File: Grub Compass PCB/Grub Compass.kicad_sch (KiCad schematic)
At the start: 28 parts, among them J1 USB_C_Receptacle_USB2.0_16P, M1 Motor_Servo, Q1 IRLML6302TRPBF, SW1 TS-1088-AR02016, SW2 TS-1088-AR02016, U1 ESP32-C3-WROOM-02, U2 AMS1117-3.3, U3 BC-4-3PD, U4 MCP73831-2-OT

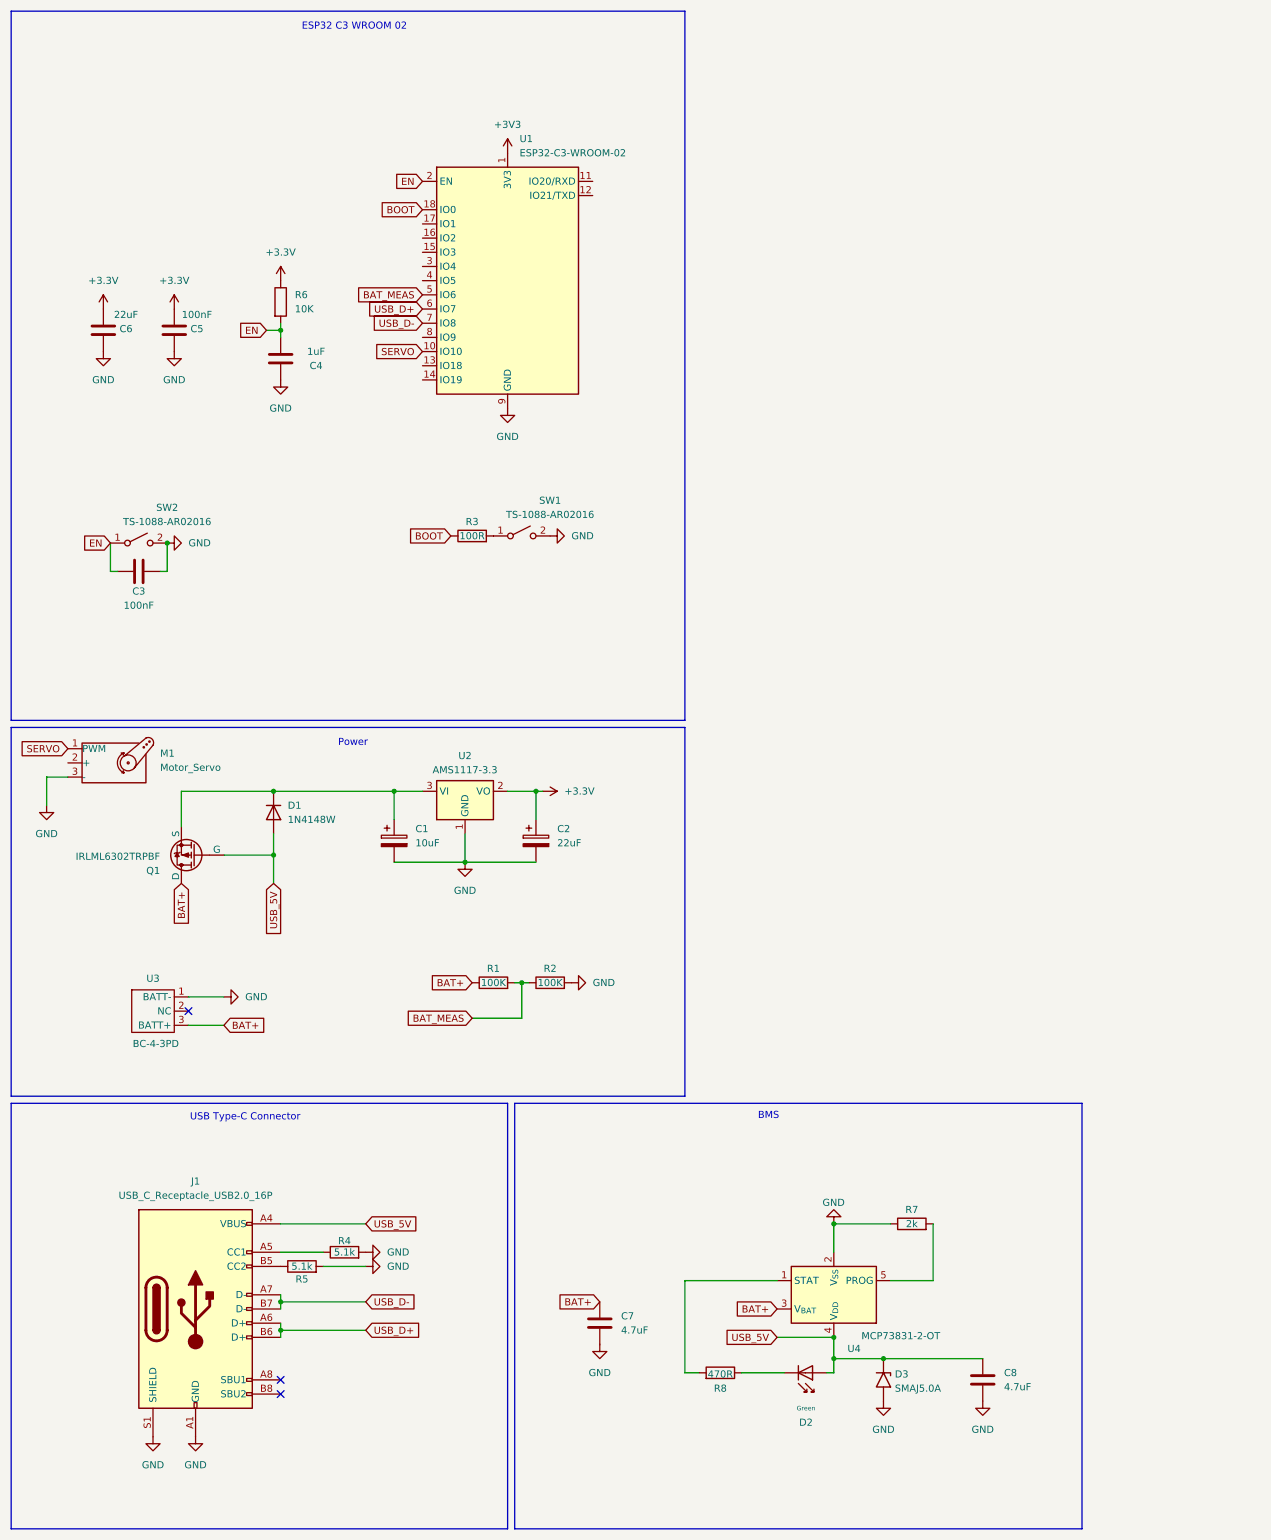
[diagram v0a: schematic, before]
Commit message: Day 3 update
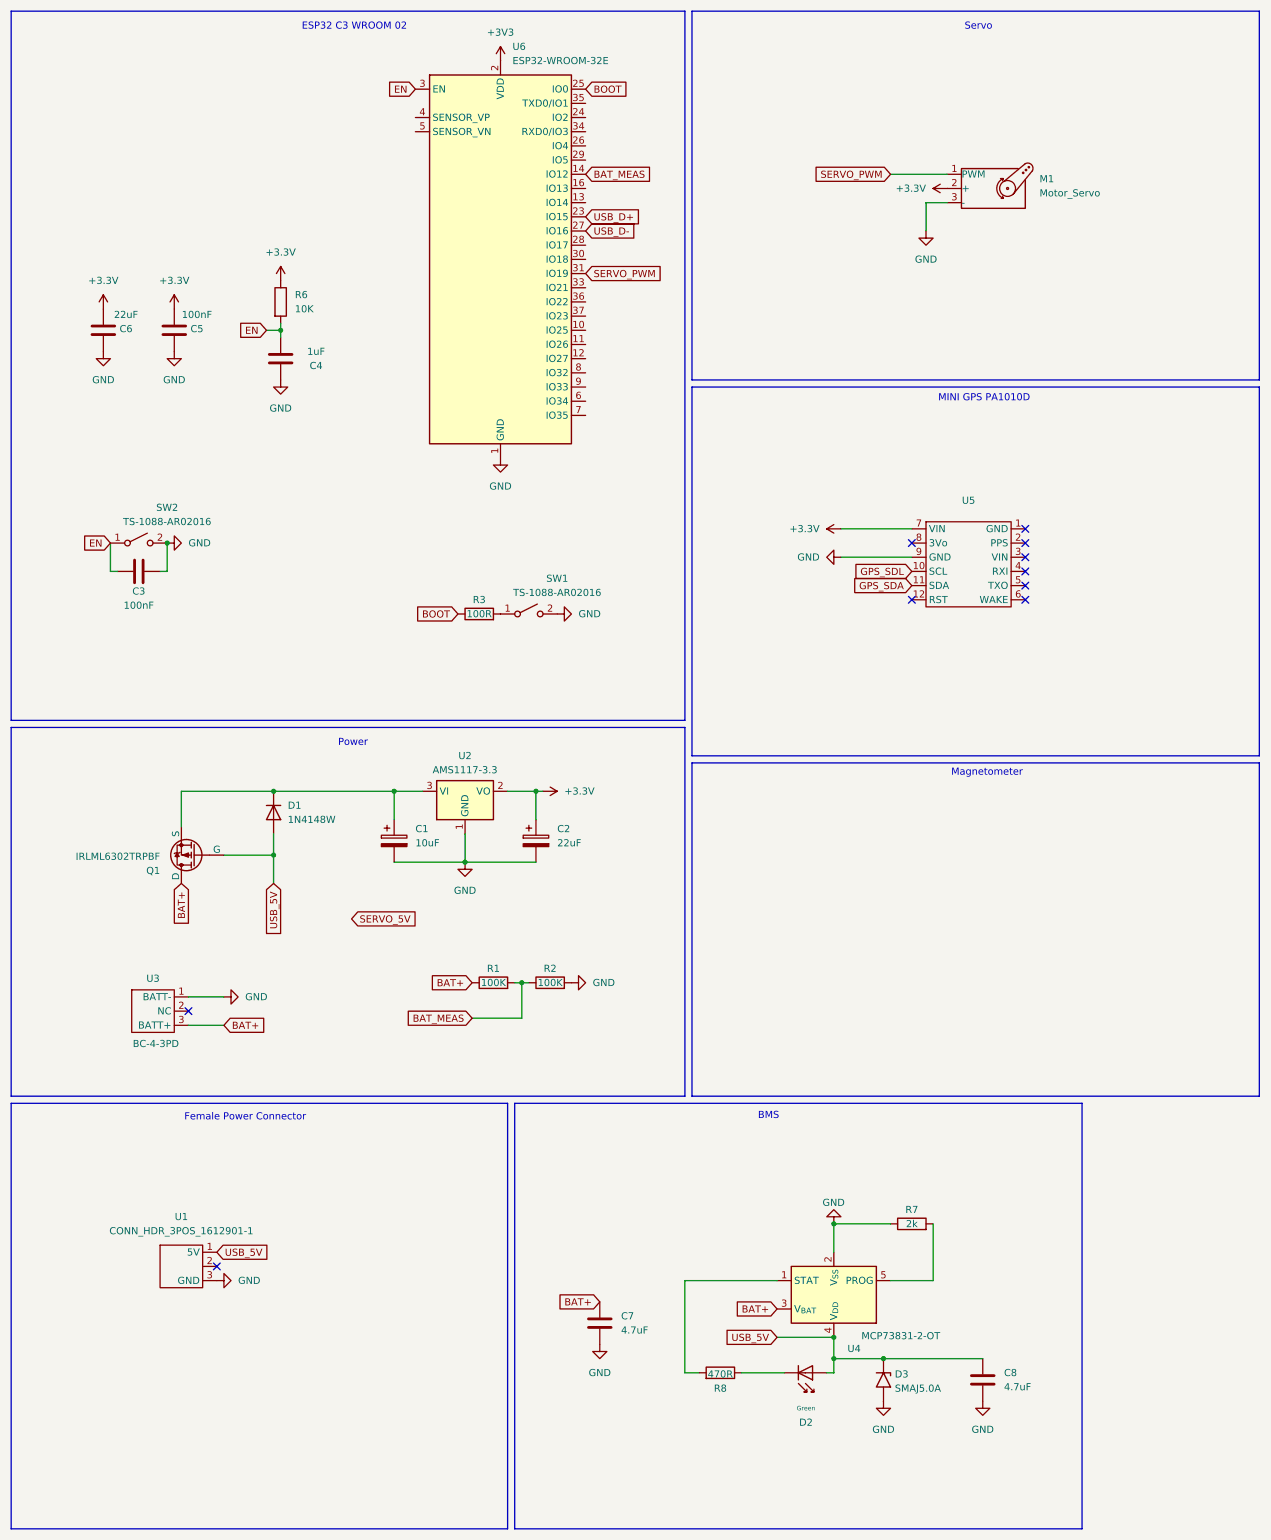
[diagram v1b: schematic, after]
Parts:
- removed J1: USB_C_Receptacle_USB2.0_16P, symbol Connector:USB_C_Receptacle_USB2.0_16P
- removed R4, R5: 5.1k, Resistor_SMD:R_0201_0603Metric, symbol Device:R
- removed U1: ESP32-C3-WROOM-02, RF_Module:ESP32-C3-WROOM-02, symbol RF_Module:ESP32-C3-WROOM-02
- added U1: CONN_HDR_3POS_1612901-1, symbol grubCompass:CONN_HDR_3POS_1612898-1
- added U5: ~, symbol grubCompass:MINI_GPS_PA1010D_STEMMA_QT
- added U6: ESP32-WROOM-32E, RF_Module:ESP32-WROOM-32D, symbol RF_Module:ESP32-WROOM-32E
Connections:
- net +3.3V: now also M1.2 (+), U5.7 (VIN)
- net +3V3: now also U6.2 (VDD)
- net BAT_MEAS: now also U6.14 (IO12)
- net BOOT: now also U6.25 (IO0)
- net EN: now also U6.3 (EN)
- net GND: now also U1.3 (GND), U5.9 (GND), U6.1 (GND), U6.15 (GND), U6.38 (GND), U6.39 (GND)
- net USB_5V: now also U1.1 (5V)
- net USB_D+: now also U6.23 (IO15)
- net USB_D-: now also U6.27 (IO16)
- net SERVO renamed SERVO_PWM
- net SERVO_PWM: now also U6.31 (IO19)
- new net GPS_SDA: U5.11 (SDA)
- new net GPS_SDL: U5.10 (SCL)
- no-connect marks 3 -> 10
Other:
- note added: "Female Power Connector"
- note added: "MINI GPS PA1010D"
- note added: "Magnetometer"
- note added: "Servo"
- note removed: "USB Type-C Connector"
- moved on the sheet: M1, R3, SW1
